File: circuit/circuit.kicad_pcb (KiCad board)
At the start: 2 copper layers, 55.1 x 20 mm, 33 parts, among them J1 USB_A, U1 RP2040, U2 AMS1117-3.3, U3 W25Q32JVSS, U4 W25Q32JVSS, Y1 12MHz

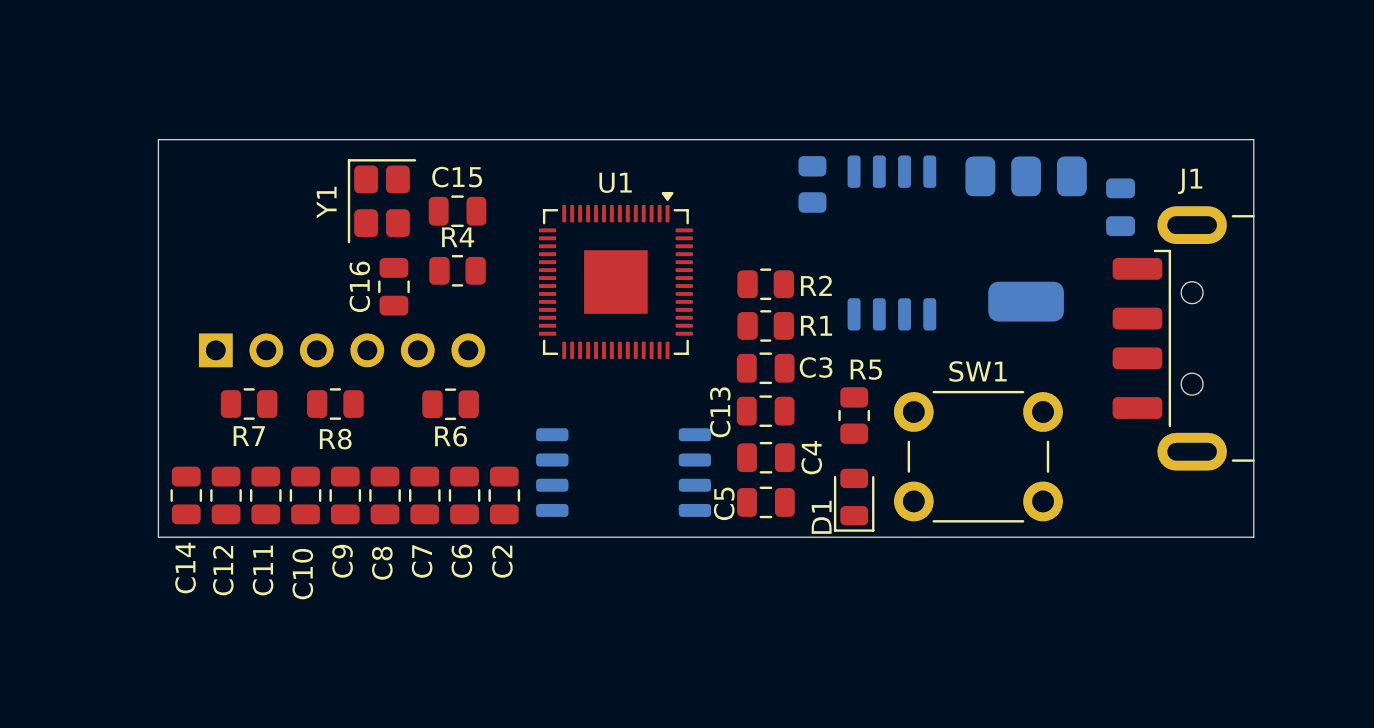
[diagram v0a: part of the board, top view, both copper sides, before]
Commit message: finalize PCB
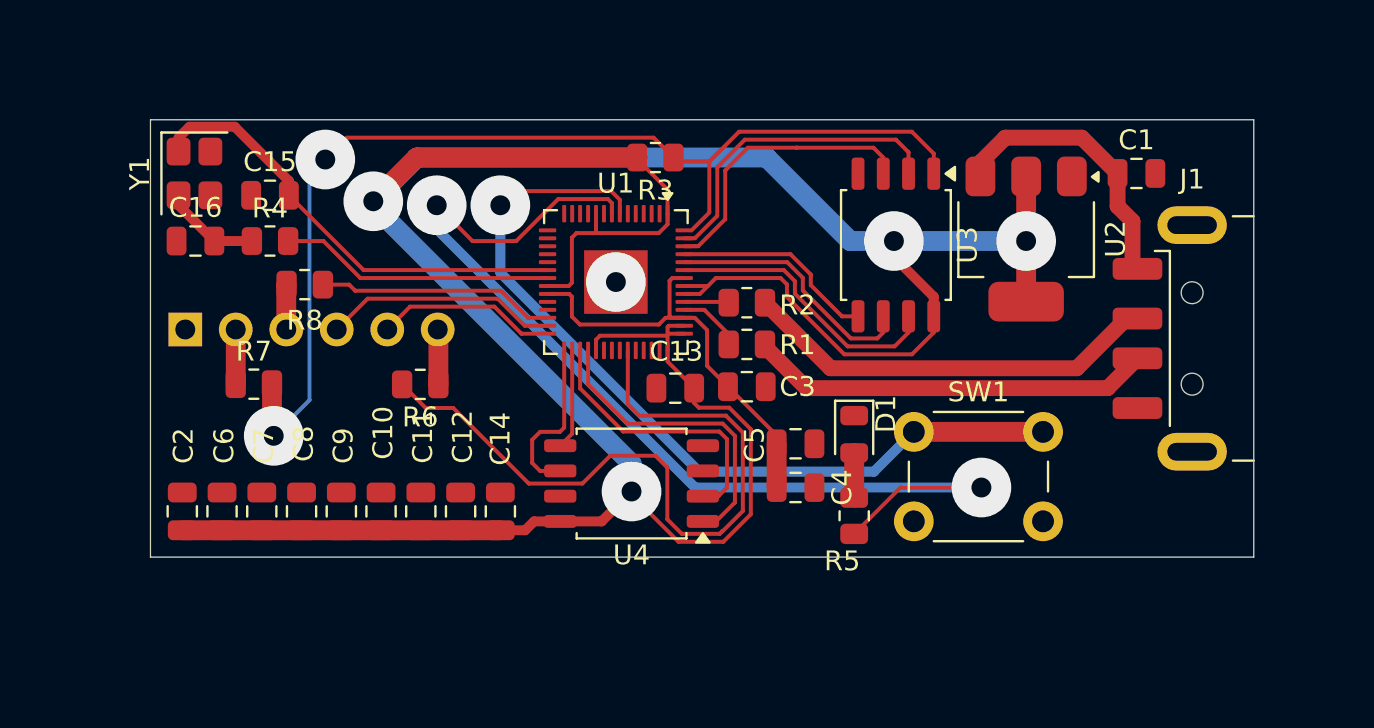
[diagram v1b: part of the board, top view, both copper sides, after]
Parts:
- C1, R3, U2, U3, U4: moved to F.Cu
- moved C2 16.2 mm to (120.4, 106.6), turned to 90 degrees
- moved C14 15.8 mm to (136.4, 106.6), turned to 90 degrees
- moved C6 12.2 mm to (122.4, 106.6), turned to 90 degrees
- moved C12 11.8 mm to (134.4, 106.6), turned to 90 degrees
- moved C16 10.2 mm to (121.1, 93.0), turned to 0 degrees
- moved R4 9.55 mm to (124.8, 93.0)
- moved Y1 9.54 mm to (121.0, 89.6)
- moved C15 9.47 mm to (124.8, 90.7)
- moved C7 8.24 mm to (124.4, 106.6), turned to 90 degrees
- moved R3 8.01 mm to (144.2, 88.8), turned to 180 degrees
- moved C11 7.84 mm to (132.4, 106.6), turned to 90 degrees
- moved R8 6.20 mm to (126.6, 95.2)
- moved R5 5.04 mm to (154.2, 106.8), turned to 90 degrees
- moved C13 4.70 mm to (145.2, 100.4), turned to 180 degrees
- moved C8 4.28 mm to (126.4, 106.6), turned to 90 degrees
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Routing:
- net +3V3: track 0.00 -> 160.6 mm, vias 0 -> 4
- net /DBG_BOOT: track 0.00 -> 54.7 mm, vias 0 -> 2
- net /IO_LED: track 0.00 -> 52.0 mm, vias 0 -> 2
- net /IO_BTN: track 0.00 -> 43.0 mm, vias 0 -> 1
- net /DBG_LED: track 0.00 -> 36.5 mm
- net /XIN: track 0.00 -> 22.9 mm
- net +1V1: track 0.00 -> 22.4 mm
- net Net-(J1-D-): track 0.00 -> 20.6 mm
- net Net-(J1-D+): track 0.00 -> 20.2 mm
- net /PMEM_IO1: track 0.00 -> 15.7 mm
- net /DMEM_CS: track 0.00 -> 15.2 mm
- net /PMEM_IO3: track 0.00 -> 14.3 mm
- net /DMEM_DO: track 0.00 -> 14.2 mm
- net VBUS: track 0.00 -> 14.1 mm
- net /XOUT: track 0.00 -> 13.8 mm
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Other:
- board size 55.1 x 20 mm -> 55.5 x 22 mm
